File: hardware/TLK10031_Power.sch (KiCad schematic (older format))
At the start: 45 parts, among them U22 TLK10031

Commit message: Added Power/Protection Circuit
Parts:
- C1205: renamed from C161; Description (none) -> CAP CER 0.1UF 6.3V X5R 0201; Populate for CLG484(Z-7012s/Z-7015) (none) -> 1; Populate for SBGA485(Z-7030) (none) -> 1
- C1206: renamed from C162; Description (none) -> CAP CER 0.1UF 6.3V X5R 0201; Populate for CLG484(Z-7012s/Z-7015) (none) -> 1; Populate for SBGA485(Z-7030) (none) -> 1
- C1207: renamed from C163; Description (none) -> CAP CER 0.1UF 6.3V X5R 0201; Populate for CLG484(Z-7012s/Z-7015) (none) -> 1; Populate for SBGA485(Z-7030) (none) -> 1
- C1208: renamed from C164; Description (none) -> CAP CER 0.1UF 6.3V X5R 0201; Populate for CLG484(Z-7012s/Z-7015) (none) -> 1; Populate for SBGA485(Z-7030) (none) -> 1
- C1209: renamed from C165; Description (none) -> CAP CER 0.1UF 6.3V X5R 0201; Populate for CLG484(Z-7012s/Z-7015) (none) -> 1; Populate for SBGA485(Z-7030) (none) -> 1
- C1210: renamed from C166; Description (none) -> CAP CER 0.1UF 6.3V X5R 0201; Populate for CLG484(Z-7012s/Z-7015) (none) -> 1; Populate for SBGA485(Z-7030) (none) -> 1
- C1211: renamed from C167; Description (none) -> CAP CER 0.1UF 6.3V X5R 0201; Populate for CLG484(Z-7012s/Z-7015) (none) -> 1; Populate for SBGA485(Z-7030) (none) -> 1
- C1212: renamed from C168; Description (none) -> CAP CER 0.1UF 6.3V X5R 0201; Populate for CLG484(Z-7012s/Z-7015) (none) -> 1; Populate for SBGA485(Z-7030) (none) -> 1
- C1213: renamed from C169; Description (none) -> CAP CER 0.1UF 6.3V X5R 0201; Populate for CLG484(Z-7012s/Z-7015) (none) -> 1; Populate for SBGA485(Z-7030) (none) -> 1
- C1216: renamed from C172; Description (none) -> CAP CER 0.1UF 6.3V X5R 0201; Populate for CLG484(Z-7012s/Z-7015) (none) -> 1; Populate for SBGA485(Z-7030) (none) -> 1
- C1218: renamed from C174; Description (none) -> CAP CER 0.1UF 6.3V X5R 0201; Populate for CLG484(Z-7012s/Z-7015) (none) -> 1; Populate for SBGA485(Z-7030) (none) -> 1
- C1220: renamed from C176; Description (none) -> CAP CER 0.1UF 6.3V X5R 0201; Populate for CLG484(Z-7012s/Z-7015) (none) -> 1; Populate for SBGA485(Z-7030) (none) -> 1
- C1221: renamed from C177; Description (none) -> CAP CER 0.1UF 6.3V X5R 0201
- C1222: renamed from C178; Description (none) -> CAP CER 0.1UF 6.3V X5R 0201; Populate for CLG484(Z-7012s/Z-7015) (none) -> 1; Populate for SBGA485(Z-7030) (none) -> 1
- C1223: renamed from C179; Description (none) -> CAP CER 0.1UF 6.3V X5R 0201
- C1224: renamed from C180; Description (none) -> CAP CER 0.1UF 6.3V X5R 0201
- C1225: renamed from C181; Description (none) -> CAP CER 0.1UF 6.3V X5R 0201
- C1227: renamed from C183; Description (none) -> CAP CER 0.1UF 6.3V X5R 0201; Populate for CLG484(Z-7012s/Z-7015) (none) -> 1; Populate for SBGA485(Z-7030) (none) -> 1
- C1229: renamed from C185; Description (none) -> CAP CER 0.1UF 6.3V X5R 0201; Populate for CLG484(Z-7012s/Z-7015) (none) -> 1; Populate for SBGA485(Z-7030) (none) -> 1
- C1230: renamed from C186; Description (none) -> CAP CER 0.1UF 6.3V X5R 0201; Populate for CLG484(Z-7012s/Z-7015) (none) -> 1; Populate for SBGA485(Z-7030) (none) -> 1
- C1231: renamed from C187; Description (none) -> CAP CER 0.1UF 6.3V X5R 0201; Populate for CLG484(Z-7012s/Z-7015) (none) -> 1; Populate for SBGA485(Z-7030) (none) -> 1
- C1234: renamed from C190; Description (none) -> CAP CER 0.1UF 6.3V X5R 0201; Populate for CLG484(Z-7012s/Z-7015) (none) -> 1; Populate for SBGA485(Z-7030) (none) -> 1
- C1235: renamed from C191; Description (none) -> CAP CER 0.1UF 6.3V X5R 0201; Populate for CLG484(Z-7012s/Z-7015) (none) -> 1; Populate for SBGA485(Z-7030) (none) -> 1
- C1236: renamed from C192; Description (none) -> CAP CER 0.1UF 6.3V X5R 0201; Populate for CLG484(Z-7012s/Z-7015) (none) -> 1; Populate for SBGA485(Z-7030) (none) -> 1
- C1237: renamed from C193; Description (none) -> CAP CER 0.1UF 6.3V X5R 0201; Populate for CLG484(Z-7012s/Z-7015) (none) -> 1; Populate for SBGA485(Z-7030) (none) -> 1
- C1238: renamed from C194; Description (none) -> CAP CER 0.1UF 6.3V X5R 0201; Populate for CLG484(Z-7012s/Z-7015) (none) -> 1; Populate for SBGA485(Z-7030) (none) -> 1
- renumbered C157 to C1201, C158 to C1202, C159 to C1203, C160 to C1204, C170 to C1214, C171 to C1215, C173 to C1217, C175 to C1219, C182 to C1226, C184 to C1228, C188 to C1232, C189 to C1233, R80 to R1201, R81 to R1202, R82 to R1203, R83 to R1204, R84 to R1205, R85 to R1206, U22 to U1201

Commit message: Length matched DDR3 Memory again.
Forgot to keep enough space between the traces and between the meander waves.

Also, I switched to Kicad 5.0 RC2.

Swaped a few ddr signals.
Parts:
- C1201, C1202, C1203, C1204, C1205, C1206, C1207, C1208, C1209, C1210, C1211, C1212, C1213, C1214, C1215, C1216, C1217, C1218, C1219, C1220, C1221, C1222, C1223, C1224, C1225, C1226, C1227, C1228, C1229, C1230, C1231, C1232, C1233, C1234, C1235, C1236, C1237, C1238: symbol C_Small -> device:C_Small
- R1201, R1202, R1203, R1204, R1205, R1206: symbol R_Small -> device:R_Small
- U1201: symbol TLK10031 -> tlk10031:TLK10031
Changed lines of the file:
@@
-EESchema Schematic File Version 2
-LIBS:zynq_board-rescue
-LIBS:power
-LIBS:device
-LIBS:transistors
-LIBS:conn
-LIBS:linear
-LIBS:regul
-LIBS:74xx
-LIBS:cmos4000
-LIBS:adc-dac
-LIBS:memory
-LIBS:xilinx
-LIBS:microcontrollers
-LIBS:dsp
-LIBS:microchip
-LIBS:analog_switches
-LIBS:motorola
-LIBS:texas
-LIBS:intel
-LIBS:audio
-LIBS:interface
-LIBS:digital-audio
-LIBS:philips
-LIBS:display
-LIBS:cypress
-LIBS:siliconi
-LIBS:opto
-LIBS:atmel
-LIBS:contrib
-LIBS:valves
-LIBS:xilinx_zynq_clg485
-LIBS:SFP_plus
-LIBS:ael2005
-LIBS:diff_osc
-LIBS:si53340
-LIBS:usb3320
-LIBS:nx5p3090
-LIBS:smp1255putg
-LIBS:osc
-LIBS:ddr
-LIBS:misc
-LIBS:tlk10031
-LIBS:lshm-150-xxx-x-dv-a-s
-LIBS:sn74axc8t245
-LIBS:sn74lvc2t45
-LIBS:dmf05lcflp
-LIBS:bss138ps
-LIBS:max14854
-LIBS:switches
-LIBS:ft234xd
-LIBS:sn74lv1t126
-LIBS:emif06-msd02n16
-LIBS:cat24c02tdi-gt3
-LIBS:power_symbols
-LIBS:ti_power_modules
-LIBS:mdr20
-LIBS:dm3cs
-LIBS:lsf0102
-LIBS:dmp3056l
+EESchema Schematic File Version 4
 LIBS:zynq_board-cache
-EELAYER 25 0
+EELAYER 26 0
 EELAYER END
 $Descr A4 11693 8268
@@
 $EndDescr
 $Comp
-L TLK10031 U1201
+L tlk10031:TLK10031 U1201
 U 2 1 5ACA3B74
 P 5550 1950
@@
 $EndComp
 $Comp
-L GND #PWR0131
+L power1:GND #PWR0131
 U 1 1 5ACA4579
 P 5450 2800
@@
 $EndComp
 $Comp
-L +1V0 #PWR0132
+L power1:+1V0 #PWR0132
 U 1 1 5ACA5A88
 P 2150 3750
@@
 1V5 or 1V8
 $Comp
-L C_Small C1201
+L device:C_Small C1201
 U 1 1 5ADD7A0B
 P 950 4350
@@
 $EndComp
 $Comp
-L C_Small C1203
+L device:C_Small C1203
 U 1 1 5ADFAF48
 P 1300 4350
@@
 $EndComp
 $Comp
-L C_Small C1205
+L device:C_Small C1205
 U 1 1 5ADFAFDF
 P 1750 4350
@@
 $EndComp
 $Comp
-L C_Small C1207
+L device:C_Small C1207
 U 1 1 5ADFC071
 P 2050 4350
@@
 $EndComp
 $Comp
-L C_Small C1209
+L device:C_Small C1209
 U 1 1 5ADFC0B6
 P 2350 4350
@@
 $EndComp
 $Comp
-L C_Small C1211
+L device:C_Small C1211
 U 1 1 5ADFC1D4
 P 2650 4350
@@
 $EndComp
 $Comp
-L C_Small C1212
+L device:C_Small C1212
 U 1 1 5ADFC1DF
 P 2950 4350
@@
 $EndComp
 $Comp
-L C_Small C1213
+L device:C_Small C1213
 U 1 1 5ADFC1EA
 P 3250 4350
@@
 $EndComp
 $Comp
-L GND #PWR0133
+L power1:GND #PWR0133
 U 1 1 5ADFCA86
 P 2150 4650
@@
 VDDA
 $Comp
-L R_Small R1201
+L device:R_Small R1201
 U 1 1 5ADFCD86
 P 2150 3950
@@
 $EndComp
 $Comp
-L +1V0 #PWR0134
+L power1:+1V0 #PWR0134
 U 1 1 5AE00745
 P 2150 5200
@@
 $EndComp
 $Comp
-L C_Small C1202
+L device:C_Small C1202
 U 1 1 5AE00750
 P 950 5800
@@
 $EndComp
 $Comp
-L C_Small C1204
+L device:C_Small C1204
 U 1 1 5AE0075B
 P 1300 5800
@@
 $EndComp
 $Comp
-L C_Small C1206
+L device:C_Small C1206
 U 1 1 5AE00766
 P 1750 5800
@@
 $EndComp
 $Comp
-L C_Small C1208
+L device:C_Small C1208
 U 1 1 5AE00771
 P 2050 5800
@@
 $EndComp
 $Comp
-L C_Small C1210
+L device:C_Small C1210
 U 1 1 5AE0077C
 P 2350 5800
@@
 $EndComp
 $Comp
-L GND #PWR0135
+L power1:GND #PWR0135
 U 1 1 5AE00796
 P 2150 6100
@@
 $EndComp
 $Comp
-L R_Small R1202
+L device:R_Small R1202
 U 1 1 5AE007A2
 P 2150 5400
@@
 VDDT
 $Comp
-L +1V0 #PWR0136
+L power1:+1V0 #PWR0136
 U 1 1 5AE013EA
 P 5350 3750
@@
 $EndComp
 $Comp
-L C_Small C1217
+L device:C_Small C1217
 U 1 1 5AE013F5
 P 4150 4350
@@
 $EndComp
 $Comp
-L C_Small C1219
+L device:C_Small C1219
 U 1 1 5AE01400
 P 4500 4350
@@
 $EndComp
 $Comp
-L C_Small C1221
+L device:C_Small C1221
 U 1 1 5AE0140B
 P 4950 4350
@@
 $EndComp
 $Comp
-L C_Small C1223
+L device:C_Small C1223
 U 1 1 5AE01416
 P 5250 4350
@@
 $EndComp
 $Comp
-L C_Small C1224
+L device:C_Small C1224
 U 1 1 5AE01421
 P 5550 4350
@@
 $EndComp
 $Comp
-L C_Small C1225
+L device:C_Small C1225
 U 1 1 5AE0142C
 P 5850 4350
@@
 $EndComp
 $Comp
-L C_Small C1227
+L device:C_Small C1227
 U 1 1 5AE01437
 P 6150 4350
@@
 $EndComp
 $Comp
-L C_Small C1229
+L device:C_Small C1229
 U 1 1 5AE01442
 P 6450 4350
@@
 $EndComp
 $Comp
-L GND #PWR0137
+L power1:GND #PWR0137
 U 1 1 5AE01466
 P 5350 4650
@@
 DVDD
 $Comp
-L R_Small R1204
+L device:R_Small R1204
 U 1 1 5AE01473
 P 5350 3950
@@
 DVDD
 $Comp
-L +1V0 #PWR0138
+L power1:+1V0 #PWR0138
 U 1 1 5AE02654
 P 8600 3750
@@
 $EndComp
 $Comp
-L C_Small C1232
+L device:C_Small C1232
 U 1 1 5AE0265F
 P 7400 4350
@@
 $EndComp
 $Comp
-L C_Small C1233
+L device:C_Small C1233
 U 1 1 5AE0266A
 P 7750 4350
@@
 $EndComp
 $Comp
-L C_Small C1234
+L device:C_Small C1234
 U 1 1 5AE02675
 P 8200 4350
@@
 $EndComp
 $Comp
-L C_Small C1235
+L device:C_Small C1235
 U 1 1 5AE02680
 P 8500 4350
@@
 $EndComp
 $Comp
-L C_Small C1236
+L device:C_Small C1236
 U 1 1 5AE0268B
 P 8800 4350
@@
 $EndComp
 $Comp
-L C_Small C1237
+L device:C_Small C1237
 U 1 1 5AE02696
 P 9100 4350
@@
 $EndComp
 $Comp
-L C_Small C1238
+L device:C_Small C1238
 U 1 1 5AE026A1
 P 9400 4350
@@
 $EndComp
 $Comp
-L GND #PWR0139
+L power1:GND #PWR0139
 U 1 1 5AE026A7
 P 8600 4650
@@
 $EndComp
 $Comp
-L R_Small R1206
+L device:R_Small R1206
 U 1 1 5AE026AF
 P 8600 3950
@@
 VDDD
 $Comp
-L C_Small C1214
+L device:C_Small C1214
 U 1 1 5AE05196
 P 3300 5800
@@
 $EndComp
 $Comp
-L C_Small C1215
+L device:C_Small C1215
 U 1 1 5AE051A1
 P 3650 5800
@@
 $EndComp
 $Comp
-L C_Small C1216
+L device:C_Small C1216
 U 1 1 5AE051AC
 P 4100 5800
@@
 $EndComp
 $Comp
-L C_Small C1218
+L device:C_Small C1218
 U 1 1 5AE051B7
 P 4400 5800
@@
 $EndComp
 $Comp
-L C_Small C1220
+L device:C_Small C1220
 U 1 1 5AE051C2
 P 4700 5800
@@
 $EndComp
 $Comp
-L C_Small C1222
+L device:C_Small C1222
 U 1 1 5AE051CD
 P 5000 5800
@@
 $EndComp
 $Comp
-L GND #PWR0140
+L power1:GND #PWR0140
 U 1 1 5AE051D3
 P 4500 6100
@@
 $EndComp
 $Comp
-L R_Small R1203
+L device:R_Small R1203
 U 1 1 5AE051DB
 P 4500 5400
@@
 	3300 5900 3300 6000
 $Comp
-L +1V8 #PWR0141
+L power1:+1V8 #PWR0141
 U 1 1 5AE05277
 P 4500 5200
@@
 VDDRA
 $Comp
-L C_Small C1226
+L device:C_Small C1226
 U 1 1 5AE06447
 P 5850 5800
@@
 $EndComp
 $Comp
-L C_Small C1228
+L device:C_Small C1228
 U 1 1 5AE06452
 P 6200 5800
@@
 $EndComp
 $Comp
-L C_Small C1230
+L device:C_Small C1230
 U 1 1 5AE0645D
 P 6650 5800
@@
 $EndComp
 $Comp
-L C_Small C1231
+L device:C_Small C1231
 U 1 1 5AE06468
 P 6950 5800
@@
 $EndComp
 $Comp
-L GND #PWR0142
+L power1:GND #PWR0142
 U 1 1 5AE06484
 P 6450 6100
@@
 $EndComp
 $Comp
-L R_Small R1205
+L device:R_Small R1205
 U 1 1 5AE0648C
 P 6450 5400
@@
 	5850 5900 5850 6000
 $Comp
-L +1V8 #PWR0143
+L power1:+1V8 #PWR0143
 U 1 1 5AE064AC
 P 6450 5200

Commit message: Layouted most of the Power Circuit and Triggerbus Levelshifters.
Added Footprint for Tantal Caps. Modified Footprint for MDR20 Connector, SD-Card.

Fixed Symbol and Circuit for Power Supervisor/Delay IC.

Also fixed some smaller things in the schematics.
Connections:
- wire segments 123 -> 261

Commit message: Improved Powerdistribution Network of the FPGA.
Also started to layout USB.
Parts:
- C1201, C1202, C1214, C1217, C1226, C1232: footprint Capacitors_SMD:C_1210 -> Capacitor_SMD:C_1210_3225Metric
- C1203, C1204, C1219, C1228, C1233: footprint Capacitors_SMD:C_0603 -> Capacitor_SMD:C_0603_1608Metric
- C1205, C1206, C1207, C1208, C1209, C1210, C1211, C1212, C1213, C1216, C1218, C1220, C1221, C1222, C1223, C1224, C1225, C1227, C1229, C1230, C1231, C1234, C1235, C1236, C1237, C1238: footprint Capacitors_SMD:C_0201 -> Capacitor_SMD:C_0201_0603Metric
- C1215: footprint Capacitors_SMD:C_0603 -> Capacitor_SMD:C_0603_1608Metric_Pad0.99x1.00mm_HandSolder

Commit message: Fixed Schematic Symbols
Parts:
- C1201, C1202, C1203, C1204, C1205, C1206, C1207, C1208, C1209, C1210, C1211, C1212, C1213, C1214, C1215, C1216, C1217, C1218, C1219, C1220, C1221, C1222, C1223, C1224, C1225, C1226, C1227, C1228, C1229, C1230, C1231, C1232, C1233, C1234, C1235, C1236, C1237, C1238: symbol device:C_Small -> Device:C_Small
- R1201, R1202, R1203, R1204, R1205, R1206: symbol device:R_Small -> Device:R_Small
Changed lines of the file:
@@
 $Descr A4 11693 8268
 encoding utf-8
-Sheet 12 22
+Sheet 12 21
 Title ""
 Date ""
@@
 $EndComp
 $Comp
-L power1:GND #PWR0131
+L power:GND #PWR0131
 U 1 1 5ACA4579
 P 5450 2800
@@
 $EndComp
 $Comp
-L power1:+1V0 #PWR0132
+L power:+1V0 #PWR0132
 U 1 1 5ACA5A88
 P 2150 3750
@@
 1V5 or 1V8
 $Comp
-L device:C_Small C1201
+L Device:C_Small C1201
 U 1 1 5ADD7A0B
 P 950 4350
@@
 $EndComp
 $Comp
-L device:C_Small C1203
+L Device:C_Small C1203
 U 1 1 5ADFAF48
 P 1300 4350
@@
 $EndComp
 $Comp
-L device:C_Small C1205
+L Device:C_Small C1205
 U 1 1 5ADFAFDF
 P 1750 4350
@@
 $EndComp
 $Comp
-L device:C_Small C1207
+L Device:C_Small C1207
 U 1 1 5ADFC071
 P 2050 4350
@@
 $EndComp
 $Comp
-L device:C_Small C1209
+L Device:C_Small C1209
 U 1 1 5ADFC0B6
 P 2350 4350
@@
 $EndComp
 $Comp
-L device:C_Small C1211
+L Device:C_Small C1211
 U 1 1 5ADFC1D4
 P 2650 4350
@@
 $EndComp
 $Comp
-L device:C_Small C1212
+L Device:C_Small C1212
 U 1 1 5ADFC1DF
 P 2950 4350
@@
 $EndComp
 $Comp
-L device:C_Small C1213
+L Device:C_Small C1213
 U 1 1 5ADFC1EA
 P 3250 4350
@@
 $EndComp
 $Comp
-L power1:GND #PWR0133
+L power:GND #PWR0133
 U 1 1 5ADFCA86
 P 2150 4650
@@
 VDDA
 $Comp
-L device:R_Small R1201
+L Device:R_Small R1201
 U 1 1 5ADFCD86
 P 2150 3950
@@
 $EndComp
 $Comp
-L power1:+1V0 #PWR0134
+L power:+1V0 #PWR0134
 U 1 1 5AE00745
 P 2150 5200
@@
 $EndComp
 $Comp
-L device:C_Small C1202
+L Device:C_Small C1202
 U 1 1 5AE00750
 P 950 5800
@@
 $EndComp
 $Comp
-L device:C_Small C1204
+L Device:C_Small C1204
 U 1 1 5AE0075B
 P 1300 5800
@@
 $EndComp
 $Comp
-L device:C_Small C1206
+L Device:C_Small C1206
 U 1 1 5AE00766
 P 1750 5800
@@
 $EndComp
 $Comp
-L device:C_Small C1208
+L Device:C_Small C1208
 U 1 1 5AE00771
 P 2050 5800
@@
 $EndComp
 $Comp
-L device:C_Small C1210
+L Device:C_Small C1210
 U 1 1 5AE0077C
 P 2350 5800
@@
 $EndComp
 $Comp
-L power1:GND #PWR0135
+L power:GND #PWR0135
 U 1 1 5AE00796
 P 2150 6100
@@
 $EndComp
 $Comp
-L device:R_Small R1202
+L Device:R_Small R1202
 U 1 1 5AE007A2
 P 2150 5400
@@
 VDDT
 $Comp
-L power1:+1V0 #PWR0136
+L power:+1V0 #PWR0136
 U 1 1 5AE013EA
 P 5350 3750
@@
 $EndComp
 $Comp
-L device:C_Small C1217
+L Device:C_Small C1217
 U 1 1 5AE013F5
 P 4150 4350
@@
 $EndComp
 $Comp
-L device:C_Small C1219
+L Device:C_Small C1219
 U 1 1 5AE01400
 P 4500 4350
@@
 $EndComp
 $Comp
-L device:C_Small C1221
+L Device:C_Small C1221
 U 1 1 5AE0140B
 P 4950 4350
@@
 $EndComp
 $Comp
-L device:C_Small C1223
+L Device:C_Small C1223
 U 1 1 5AE01416
 P 5250 4350
@@
 $EndComp
 $Comp
-L device:C_Small C1224
+L Device:C_Small C1224
 U 1 1 5AE01421
 P 5550 4350
@@
 $EndComp
 $Comp
-L device:C_Small C1225
+L Device:C_Small C1225
 U 1 1 5AE0142C
 P 5850 4350
@@
 $EndComp
 $Comp
-L device:C_Small C1227
+L Device:C_Small C1227
 U 1 1 5AE01437
 P 6150 4350
@@
 $EndComp
 $Comp
-L device:C_Small C1229
+L Device:C_Small C1229
 U 1 1 5AE01442
 P 6450 4350
@@
 $EndComp
 $Comp
-L power1:GND #PWR0137
+L power:GND #PWR0137
 U 1 1 5AE01466
 P 5350 4650
@@
 DVDD
 $Comp
-L device:R_Small R1204
+L Device:R_Small R1204
 U 1 1 5AE01473
 P 5350 3950
@@
 DVDD
 $Comp
-L power1:+1V0 #PWR0138
+L power:+1V0 #PWR0138
 U 1 1 5AE02654
 P 8600 3750
@@
 $EndComp
 $Comp
-L device:C_Small C1232
+L Device:C_Small C1232
 U 1 1 5AE0265F
 P 7400 4350
@@
 $EndComp
 $Comp
-L device:C_Small C1233
+L Device:C_Small C1233
 U 1 1 5AE0266A
 P 7750 4350
@@
 $EndComp
 $Comp
-L device:C_Small C1234
+L Device:C_Small C1234
 U 1 1 5AE02675
 P 8200 4350
@@
 $EndComp
 $Comp
-L device:C_Small C1235
+L Device:C_Small C1235
 U 1 1 5AE02680
 P 8500 4350
@@
 $EndComp
 $Comp
-L device:C_Small C1236
+L Device:C_Small C1236
 U 1 1 5AE0268B
 P 8800 4350
@@
 $EndComp
 $Comp
-L device:C_Small C1237
+L Device:C_Small C1237
 U 1 1 5AE02696
 P 9100 4350
@@
 $EndComp
 $Comp
-L device:C_Small C1238
+L Device:C_Small C1238
 U 1 1 5AE026A1
 P 9400 4350
@@
 $EndComp
 $Comp
-L power1:GND #PWR0139
+L power:GND #PWR0139
 U 1 1 5AE026A7
 P 8600 4650
@@
 $EndComp
 $Comp
-L device:R_Small R1206
+L Device:R_Small R1206
 U 1 1 5AE026AF
 P 8600 3950
@@
 VDDD
 $Comp
-L device:C_Small C1214
+L Device:C_Small C1214
 U 1 1 5AE05196
 P 3300 5800
@@
 $EndComp
 $Comp
-L device:C_Small C1215
+L Device:C_Small C1215
 U 1 1 5AE051A1
 P 3650 5800
@@
 $EndComp
 $Comp
-L device:C_Small C1216
+L Device:C_Small C1216
 U 1 1 5AE051AC
 P 4100 5800
@@
 $EndComp
 $Comp
-L device:C_Small C1218
+L Device:C_Small C1218
 U 1 1 5AE051B7
 P 4400 5800
@@
 $EndComp
 $Comp
-L device:C_Small C1220
+L Device:C_Small C1220
 U 1 1 5AE051C2
 P 4700 5800
@@
 $EndComp
 $Comp
-L device:C_Small C1222
+L Device:C_Small C1222
 U 1 1 5AE051CD
 P 5000 5800
@@
 $EndComp
 $Comp
-L power1:GND #PWR0140
+L power:GND #PWR0140
 U 1 1 5AE051D3
 P 4500 6100
@@
 $EndComp
 $Comp
-L device:R_Small R1203
+L Device:R_Small R1203
 U 1 1 5AE051DB
 P 4500 5400
@@
 	3300 5900 3300 6000
 $Comp
-L power1:+1V8 #PWR0141
+L power:+1V8 #PWR0141
 U 1 1 5AE05277
 P 4500 5200
@@
 VDDRA
 $Comp
-L device:C_Small C1226
+L Device:C_Small C1226
 U 1 1 5AE06447
 P 5850 5800
@@
 $EndComp
 $Comp
-L device:C_Small C1228
+L Device:C_Small C1228
 U 1 1 5AE06452
 P 6200 5800
@@
 $EndComp
 $Comp
-L device:C_Small C1230
+L Device:C_Small C1230
 U 1 1 5AE0645D
 P 6650 5800
@@
 $EndComp
 $Comp
-L device:C_Small C1231
+L Device:C_Small C1231
 U 1 1 5AE06468
 P 6950 5800
@@
 $EndComp
 $Comp
-L power1:GND #PWR0142
+L power:GND #PWR0142
 U 1 1 5AE06484
 P 6450 6100
@@
 $EndComp
 $Comp
-L device:R_Small R1205
+L Device:R_Small R1205
 U 1 1 5AE0648C
 P 6450 5400
@@
 	5850 5900 5850 6000
 $Comp
-L power1:+1V8 #PWR0143
+L power:+1V8 #PWR0143
 U 1 1 5AE064AC
 P 6450 5200

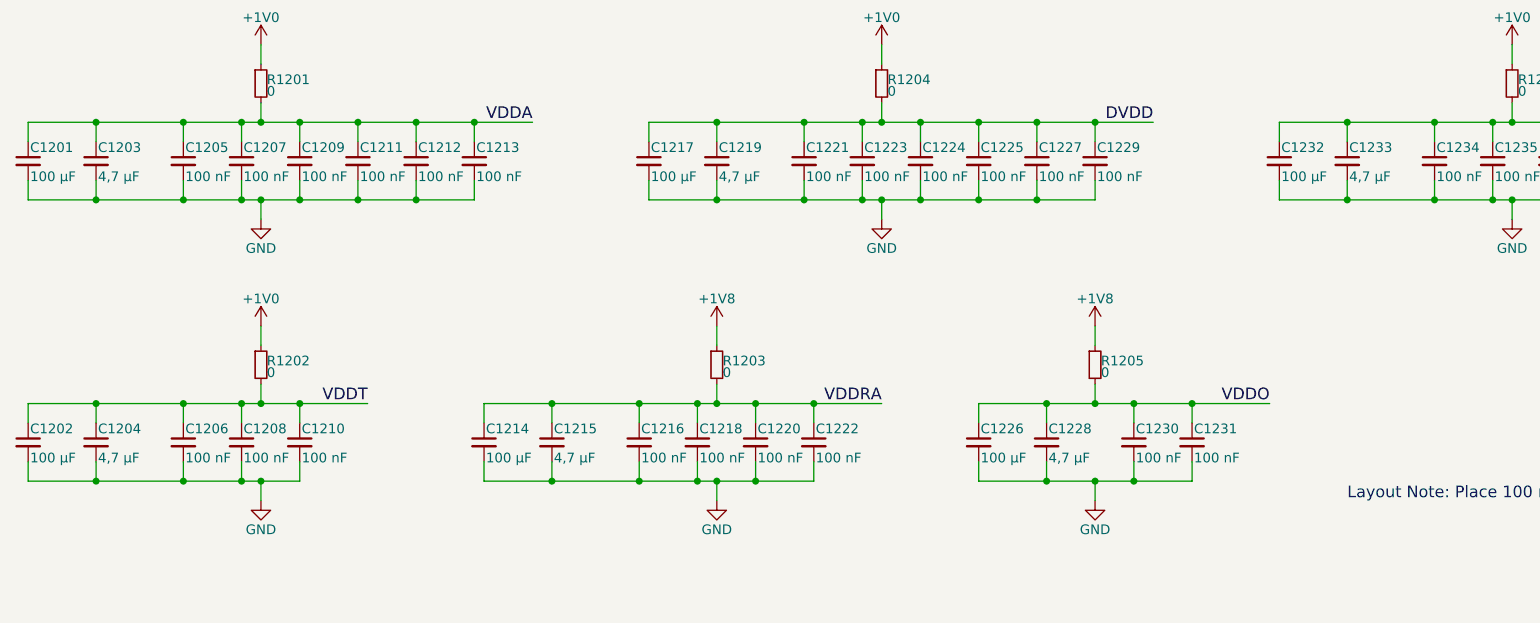
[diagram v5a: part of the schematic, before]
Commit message: WIP: TLK Powerdistribution
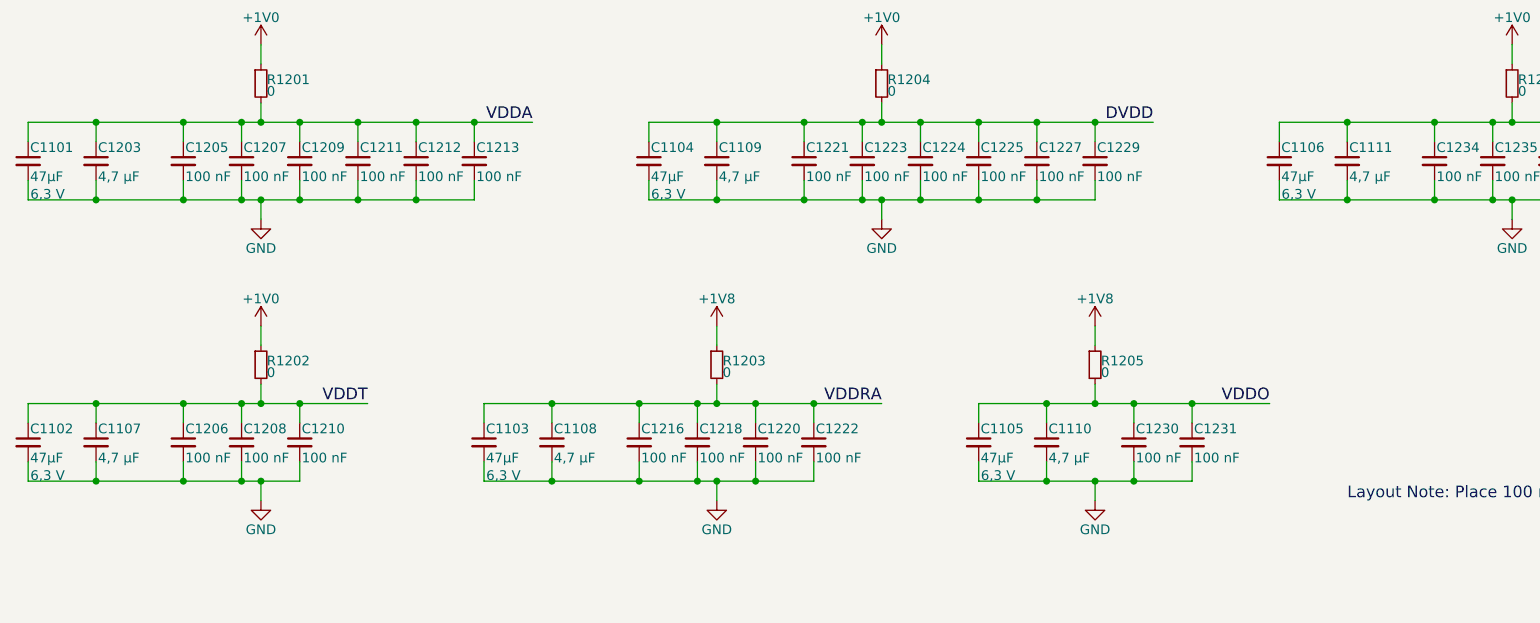
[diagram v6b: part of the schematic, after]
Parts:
- removed C1201, C1202, C1214, C1217, C1226, C1232: 100 µF, Capacitor_SMD:C_1210_3225Metric, symbol Device:C_Small
- removed C1204, C1219, C1228, C1233: 4,7 µF, Capacitor_SMD:C_0603_1608Metric, symbol Device:C_Small
- removed C1215: 4,7 µF, Capacitor_SMD:C_0603_1608Metric_Pad0.99x1.00mm_HandSolder, symbol Device:C_Small
- added C1101, C1102, C1103, C1104, C1105, C1106: 47µF, Capacitor_SMD:C_0603_1608Metric, symbol Device:C_Small
- added C1107, C1108, C1109, C1110, C1111: 4,7 µF, Capacitor_SMD:C_0603_1608Metric, symbol Device:C_Small
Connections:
- net DVDD: now also C1104.1, C1109.1
- net GND: now also C1101.2, C1102.2, C1103.2, C1104.2, C1105.2, C1106.2, C1107.2, C1108.2, C1109.2, C1110.2, C1111.2
- net VDDA: now also C1101.1
- net VDDD: now also C1106.1, C1111.1
- net VDDO: now also C1105.1, C1110.1
- net VDDRA: now also C1103.1, C1108.1
- net VDDT: now also C1102.1, C1107.1
